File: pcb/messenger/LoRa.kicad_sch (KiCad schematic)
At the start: 19 parts, among them J5 Conn_Coaxial, Q1_Xtal1 32.0MHz, U3 SX1262IMLTRT, U6 BGS12WN6E6327

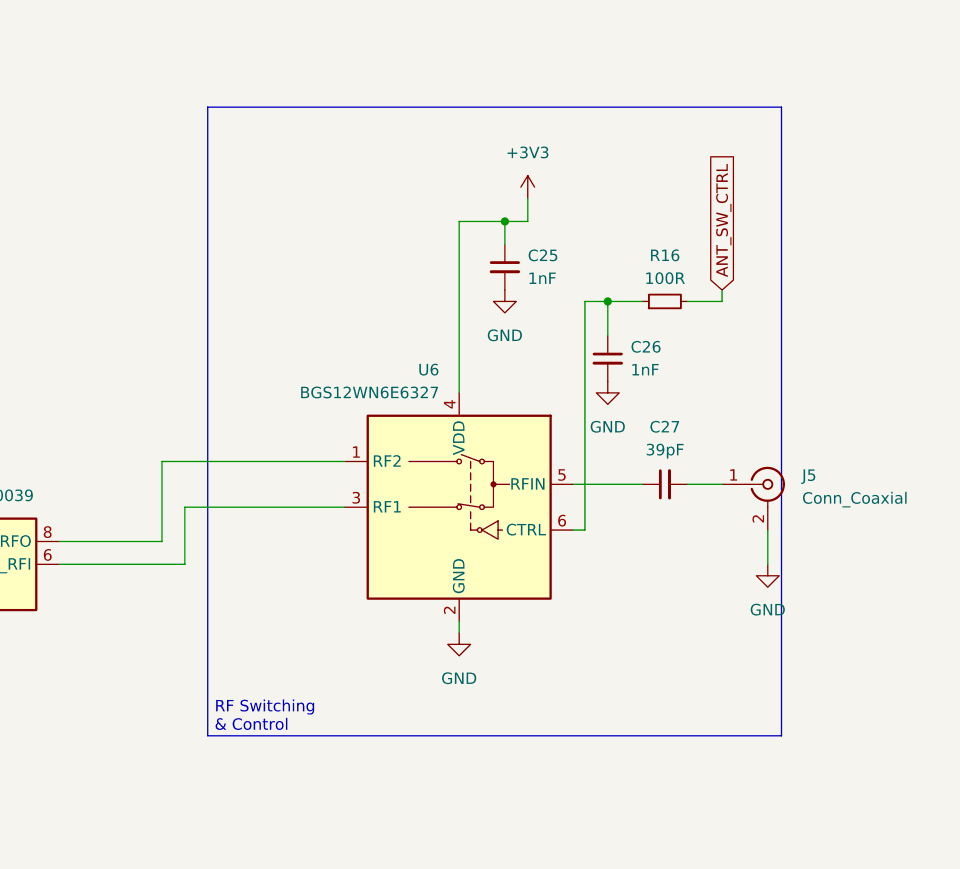
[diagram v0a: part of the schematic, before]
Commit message: still dont work
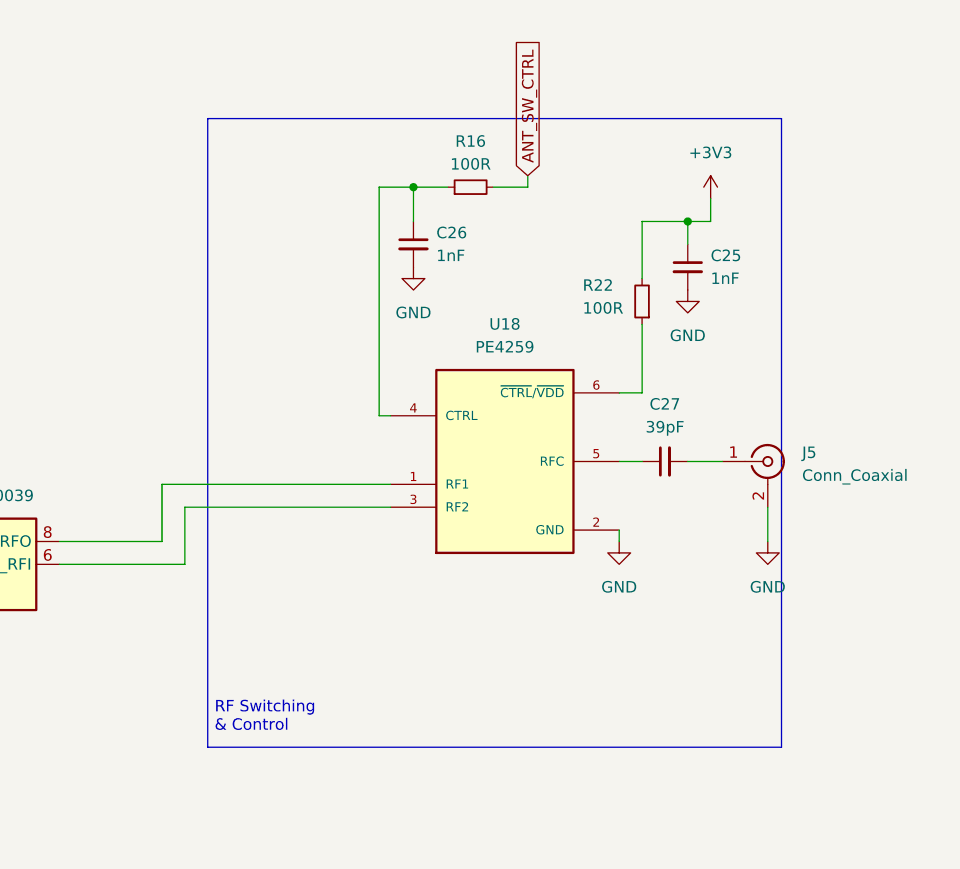
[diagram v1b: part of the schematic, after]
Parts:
- removed U6: BGS12WN6E6327, Package_LGA:Infineon_PG-TSNP-6-10_0.7x1.1mm_0.7x1.1mm_P0.4mm, symbol RF_Switch:BGS12WN6E6327
- added R22: 100R, Resistor_SMD:R_0402_1005Metric, symbol Device:R_Small
- added U18: PE4259, PE4259:SC-70-6_PSM, symbol PE4259:PE4259
- J5: footprint Connector_Coaxial:SMA_Amphenol_901-143_Horizontal -> Connector_Coaxial:U.FL_Molex_MCRF_73412-0110_Vertical
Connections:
- net +3V3: now also R22.2
- net GND: now also U18.2 (GND)
- net at FL1.6 (SW_RFI): now also U18.3 (RF2)
- net at FL1.8 (SW_RFO): now also U18.1 (RF1)
- net at C27.1: now also U18.5 (RFC)
- net at C26.1, R16.1: now also U18.4 (CTRL)
- new net: R22.1, U18.6 (~{CTRL}/~{VDD})
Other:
- moved on the sheet: C25, C26, C27, J5, R16
